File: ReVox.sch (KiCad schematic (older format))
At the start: 42 parts, among them CN1 EXPANSION_PORT, CN2 AUDIO_OUT, CN3 AUDIO_OUT, CN4 CN_RAW_DAC, U1 GAL20V8, U2 74LS273, U3 TLC272

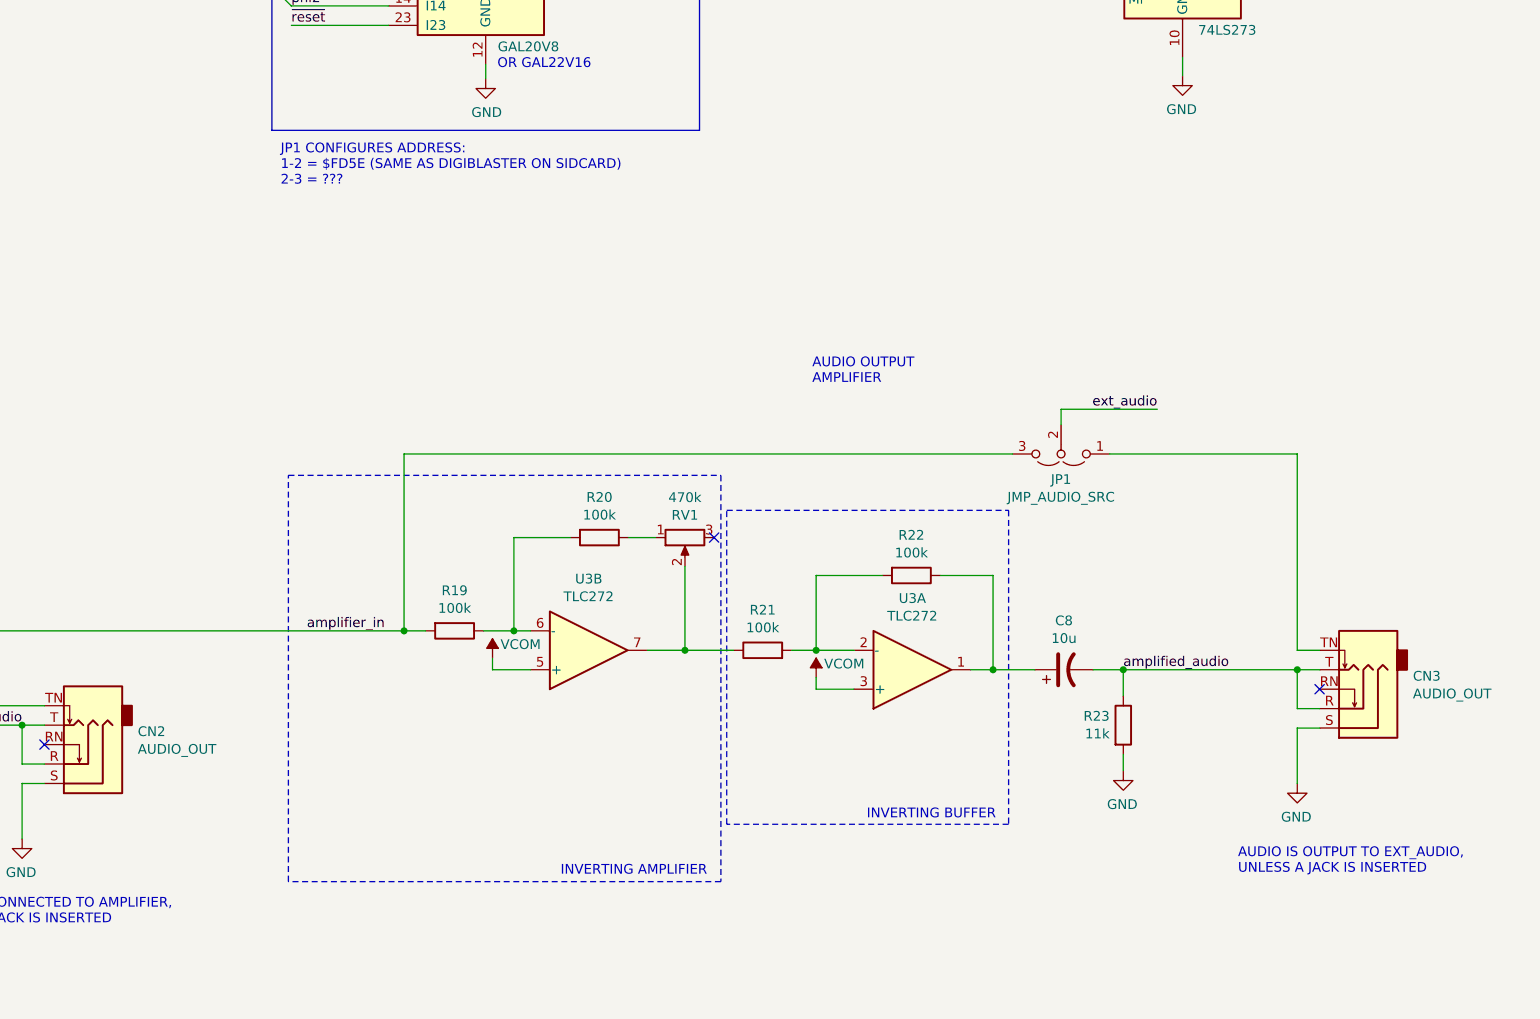
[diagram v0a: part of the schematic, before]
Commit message: Final touches
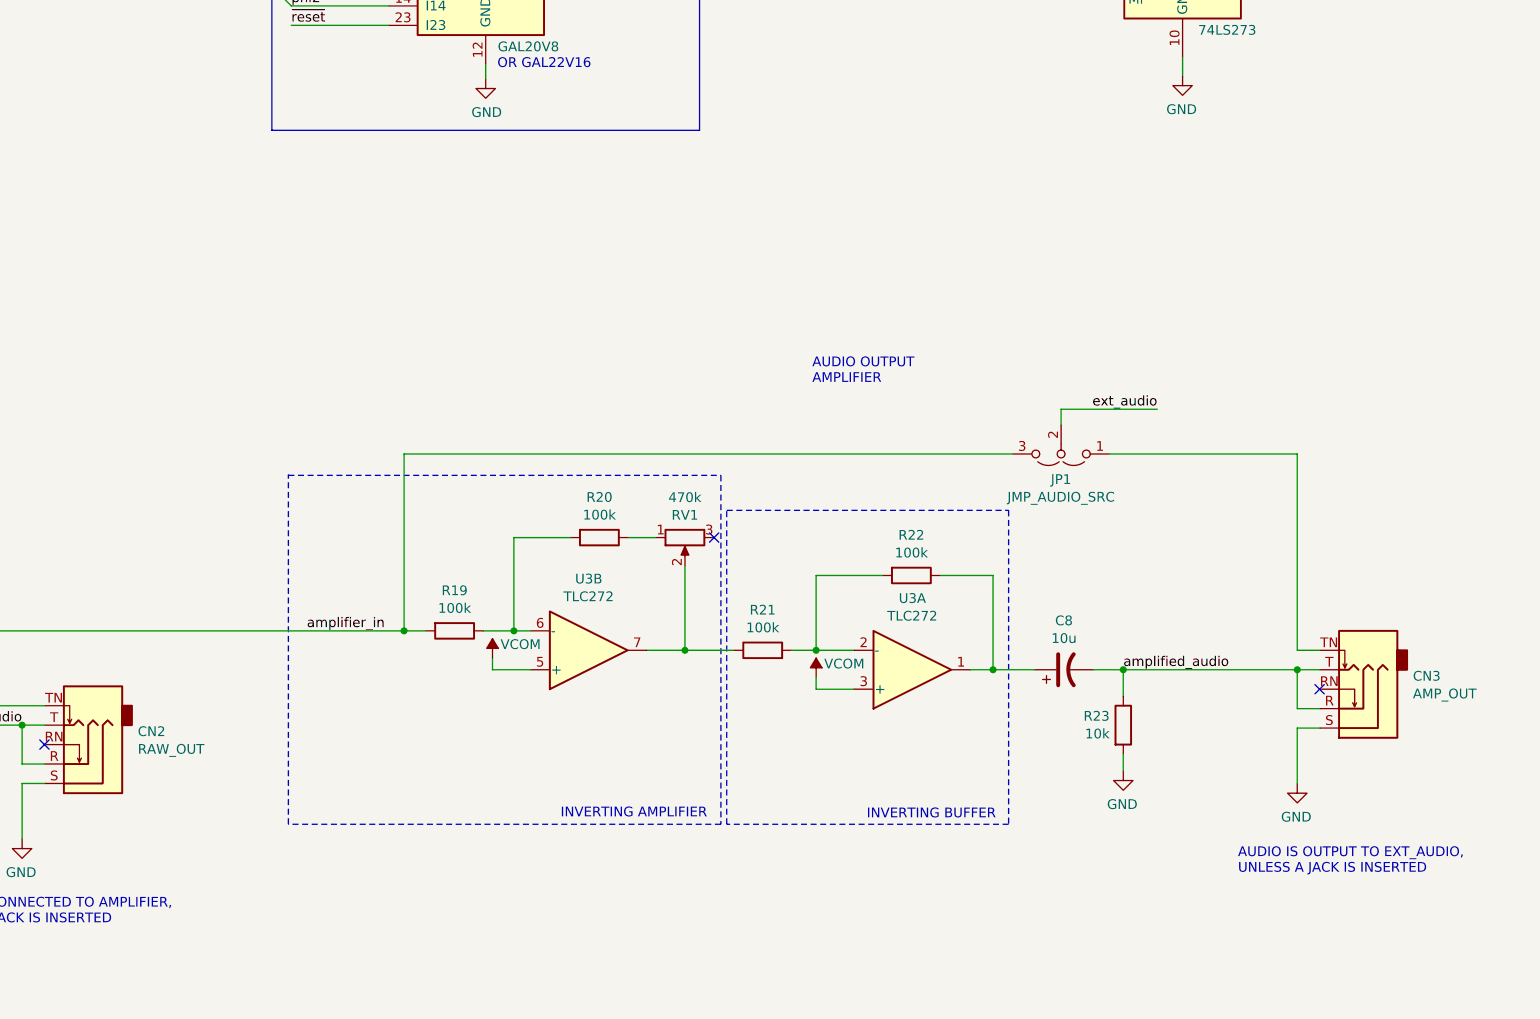
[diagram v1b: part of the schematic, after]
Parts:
- C5: Notes Optional, filters DAC output -> DAC output low-pass filter, goes to taste in the 470pF-10nF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
- C7, C8: MouserPN (none) -> 710-860010572002
- CN2: value AUDIO_OUT -> RAW_OUT
- CN3: value AUDIO_OUT -> AMP_OUT
- CN4: MouserPN (none) -> -; Notes (none) -> Mainly meant for debugging
- JP1: MouserPN (none) -> -
- R1, R10, R12, R14, R16, R2, R4, R6, R8: Notes (none) -> Exact value is not critical as long as it is exactly TWICE 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
- R11, R13, R15, R3, R5, R7, R9: Notes (none) -> Exact value is not critical as long as it is exactly HALF R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
- R19, R20: MouserPN (none) -> 603-MFR-25FTE52-11K; Notes (none) -> 1% or better
- R21, R22: Notes (none) -> 1% or better
- R23: value 11k -> 10k
- RV1: MouserPN 652-3306P-1-103 -> (none); Notes Skip if Gain control is not desired -> (none)
- U3: MouserPN (none) -> 595-TLC272BIP
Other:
- note removed: "JP1 CONFIGURES ADDRESS:\n1-2 = $FD5E (SAME AS DIGIBLASTER ON SIDCARD)\n2-3 = ???"
